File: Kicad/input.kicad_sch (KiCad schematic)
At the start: 10 parts, among them J1 AudioJack4, U17 TMUX4053DYYR, U4 OPA1656ID

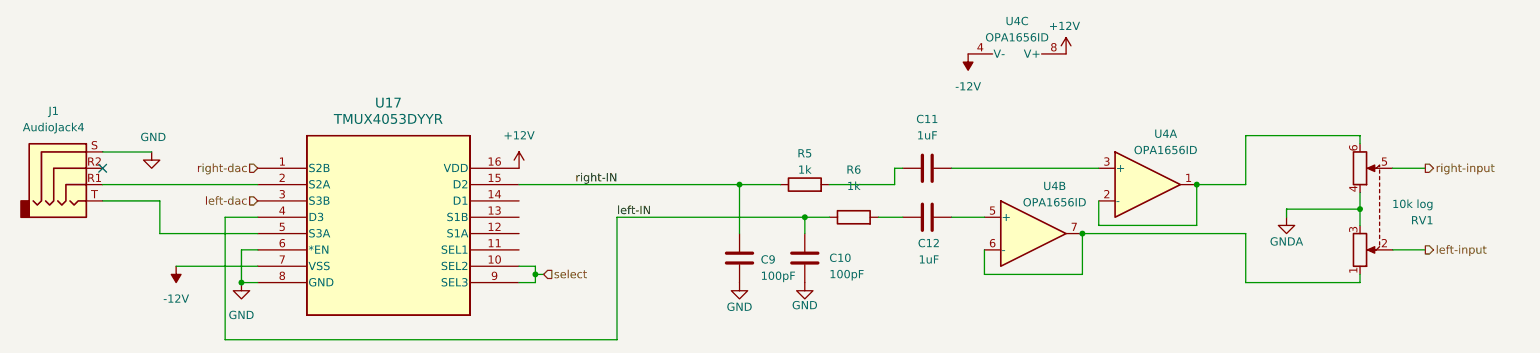
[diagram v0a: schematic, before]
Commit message: fixed issues in amp
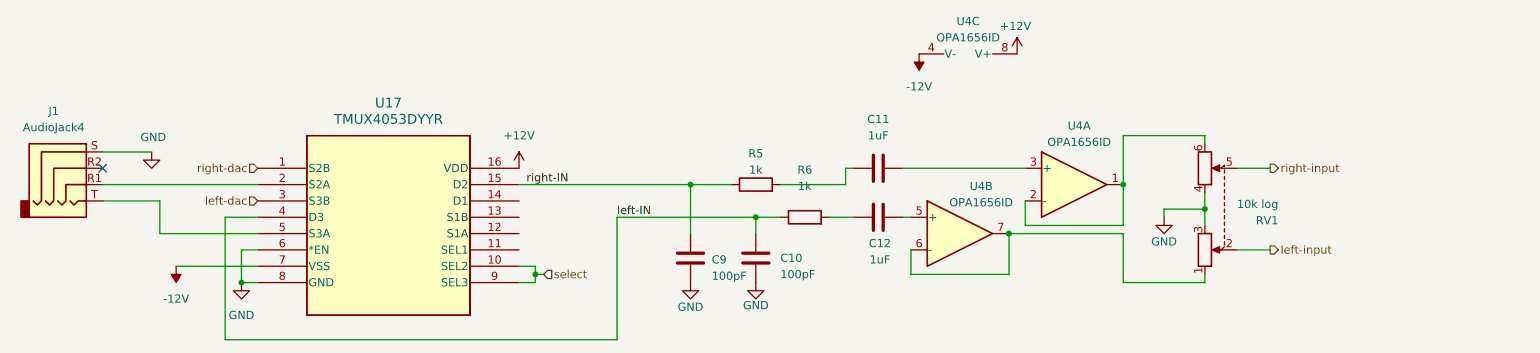
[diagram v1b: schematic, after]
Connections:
- net GNDA is gone; now on net GND: RV1.3, RV1.4
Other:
- moved on the sheet: C10, C11, C12, C9, R5, R6, RV1, U4A, U4B, U4C
